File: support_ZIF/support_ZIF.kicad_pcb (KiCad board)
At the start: 2 copper layers, 10.8 x 42.5 mm, 2 parts, among them J1 Conn_02x10_Counter_Clockwise, J2 Conn_01x05

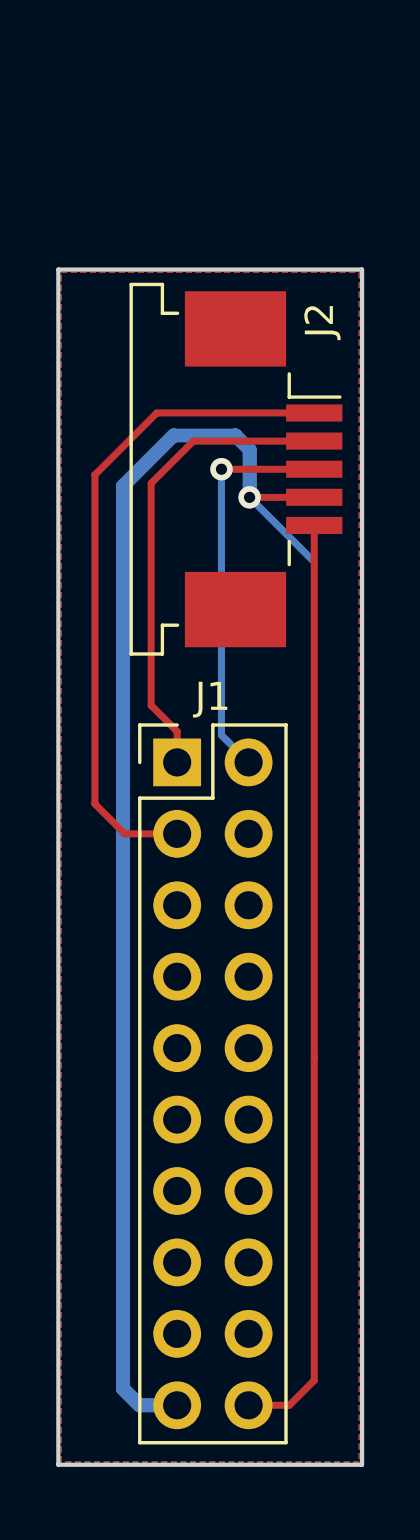
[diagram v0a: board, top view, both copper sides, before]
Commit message: 3D sandwich
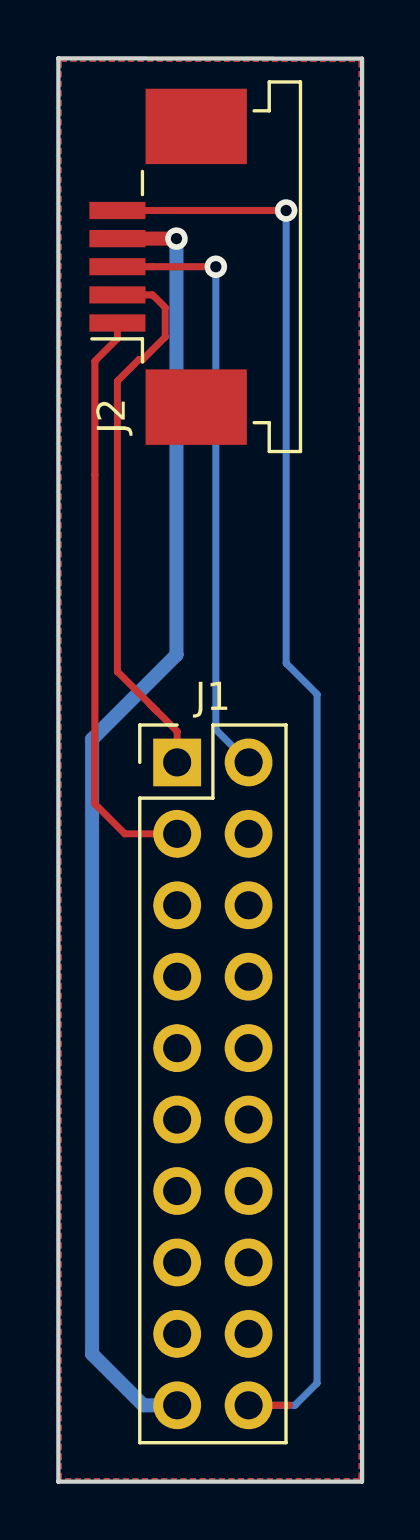
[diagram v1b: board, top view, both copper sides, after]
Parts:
- moved J2 7.96 mm to (68.4, 17.7), turned to 90 degrees
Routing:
- net /GND: track 33.1 -> 52.4 mm, vias 0 -> 1
- net /TWI_SDA: track 14.1 -> 21.6 mm
- net /TWI_CLK: track 16.7 -> 20.0 mm
- net /P0.02_AMP_OUT: track 23.8 -> 20.8 mm
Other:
- board size 10.8 x 42.5 mm -> 10.8 x 50.6 mm
